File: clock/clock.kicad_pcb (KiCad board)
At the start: 2 copper layers, 100 x 50 mm, 22 parts, among them J1 USB_OTG, J2 Barrel_Jack, U1 iv12, U2 iv12, U3 iv12, U4 iv12, U5 STM32F103C8Tx, Y1 8Mhz, Y2 32.768khz

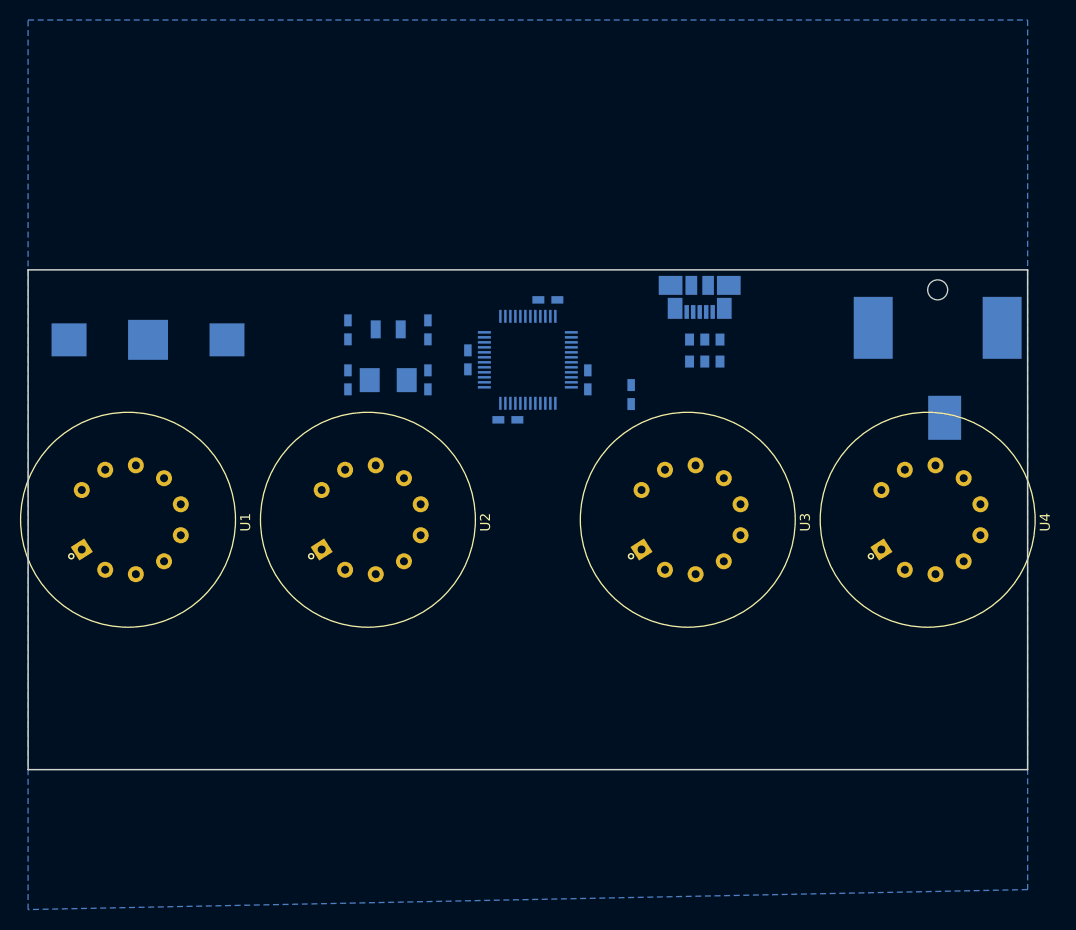
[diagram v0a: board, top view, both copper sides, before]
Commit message: Rev 1 of clock display board
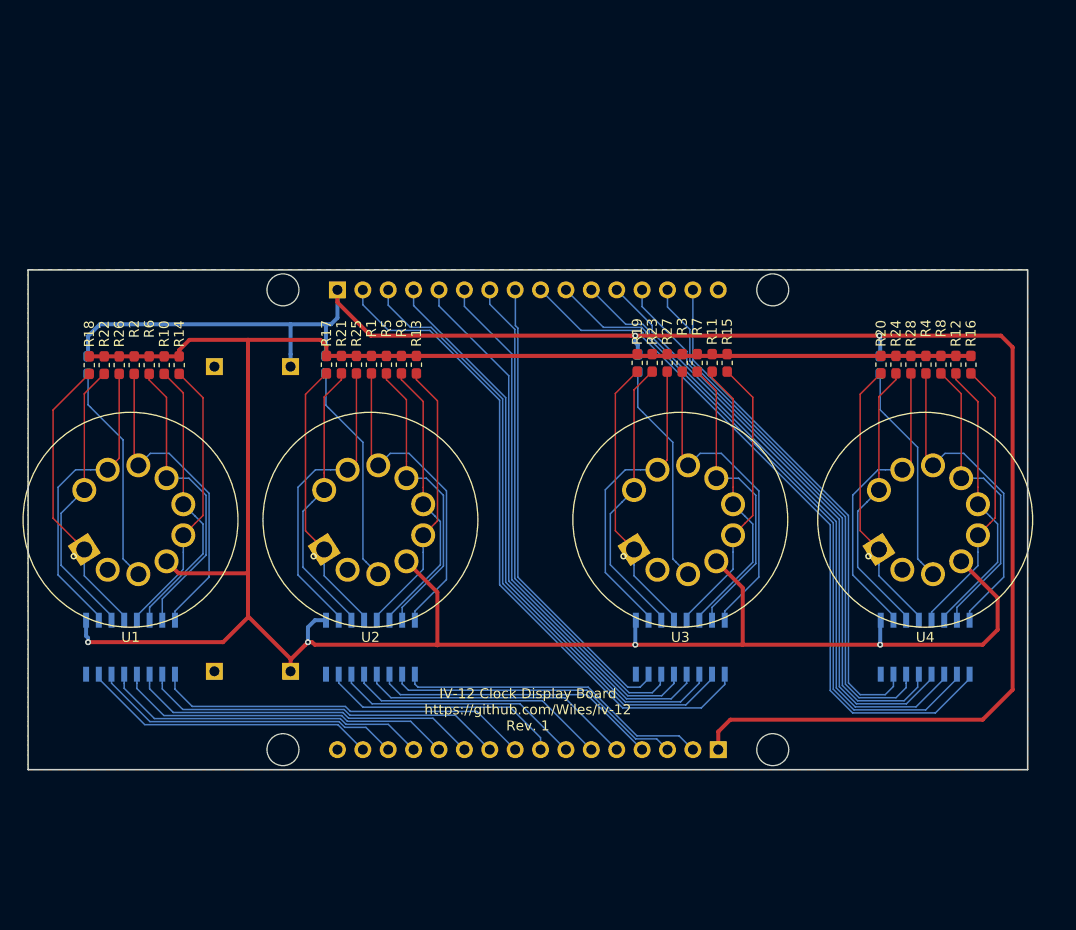
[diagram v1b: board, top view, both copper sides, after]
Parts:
- removed BT1: Battery_Cell, Battery_Holders:Keystone_3000_1x12mm-CoinCell
- removed C1, C2, C3, C4: 20p, Capacitors_SMD:C_0603_HandSoldering
- removed C5, C6, C7, C8, C9: 104, Capacitors_SMD:C_0603_HandSoldering
- removed Y1: 8Mhz, Crystals:Crystal_SMD_5032-2pin_5.0x3.2mm
- removed Y2: 32.768khz, Crystals:Crystal_SMD_3215-2pin_3.2x1.5mm
- added J3: 5v, Connector_PinHeader_2.54mm:PinHeader_1x01_P2.54mm_Vertical, B.Cu at (103.3, 111.7)
- added J4: Conn_01x01_Male, Connector_PinHeader_2.54mm:PinHeader_1x01_P2.54mm_Vertical, B.Cu at (95.6, 111.7)
- added J5: 24v, Connector_PinHeader_2.54mm:PinHeader_1x01_P2.54mm_Vertical, B.Cu at (103.3, 142.2)
- added J6: Conn_01x01_Male, Connector_PinHeader_2.54mm:PinHeader_1x01_P2.54mm_Vertical, B.Cu at (95.6, 142.2)
- added R10: 10k, Resistor_SMD:R_0603_1608Metric_Pad1.05x0.95mm_HandSolder, F.Cu at (90.6, 111.5)
- added R11: 10k, Resistor_SMD:R_0603_1608Metric_Pad1.05x0.95mm_HandSolder, F.Cu at (145.4, 111.3)
- added R12: 10k, Resistor_SMD:R_0603_1608Metric_Pad1.05x0.95mm_HandSolder, F.Cu at (169.8, 111.5)
- added R13: 10k, Resistor_SMD:R_0603_1608Metric_Pad1.05x0.95mm_HandSolder, F.Cu at (115.8, 111.5)
- added R14: 10k, Resistor_SMD:R_0603_1608Metric_Pad1.05x0.95mm_HandSolder, F.Cu at (92.1, 111.5)
- added R15: 10k, Resistor_SMD:R_0603_1608Metric_Pad1.05x0.95mm_HandSolder, F.Cu at (146.9, 111.3)
- added R16: 10k, Resistor_SMD:R_0603_1608Metric_Pad1.05x0.95mm_HandSolder, F.Cu at (171.3, 111.5)
- added R17: 10k, Resistor_SMD:R_0603_1608Metric_Pad1.05x0.95mm_HandSolder, F.Cu at (106.8, 111.5)
- added R18: 10k, Resistor_SMD:R_0603_1608Metric_Pad1.05x0.95mm_HandSolder, F.Cu at (83.1, 111.5)
- added R19: 10k, Resistor_SMD:R_0603_1608Metric_Pad1.05x0.95mm_HandSolder, F.Cu at (137.9, 111.3)
- added R20: 10k, Resistor_SMD:R_0603_1608Metric_Pad1.05x0.95mm_HandSolder, F.Cu at (162.3, 111.5)
- added R21: 10k, Resistor_SMD:R_0603_1608Metric_Pad1.05x0.95mm_HandSolder, F.Cu at (108.3, 111.5)
- added R22: 10k, Resistor_SMD:R_0603_1608Metric_Pad1.05x0.95mm_HandSolder, F.Cu at (84.6, 111.5)
- added R23: 10k, Resistor_SMD:R_0603_1608Metric_Pad1.05x0.95mm_HandSolder, F.Cu at (139.4, 111.3)
- added R24: 10k, Resistor_SMD:R_0603_1608Metric_Pad1.05x0.95mm_HandSolder, F.Cu at (163.8, 111.5)
- added R25: 10k, Resistor_SMD:R_0603_1608Metric_Pad1.05x0.95mm_HandSolder, F.Cu at (109.8, 111.5)
- added R26: 10k, Resistor_SMD:R_0603_1608Metric_Pad1.05x0.95mm_HandSolder, F.Cu at (86.1, 111.5)
- added R27: 10k, Resistor_SMD:R_0603_1608Metric_Pad1.05x0.95mm_HandSolder, F.Cu at (140.9, 111.3)
- added R28: 10k, Resistor_SMD:R_0603_1608Metric_Pad1.05x0.95mm_HandSolder, F.Cu at (165.3, 111.5)
- added R29: R_Small, Resistor_SMD:R_0603_1608Metric_Pad1.05x0.95mm_HandSolder, B.Cu at (138.0, 111.3)
- added R30: R_Small, Resistor_SMD:R_0603_1608Metric_Pad1.05x0.95mm_HandSolder, B.Cu at (106.8, 111.5)
- added R31: R_Small, Resistor_SMD:R_0603_1608Metric_Pad1.05x0.95mm_HandSolder, B.Cu at (83.0, 111.5)
- added R32: R_Small, Resistor_SMD:R_0603_1608Metric_Pad1.05x0.95mm_HandSolder, B.Cu at (162.2, 111.5)
- added R4: 10k, Resistor_SMD:R_0603_1608Metric_Pad1.05x0.95mm_HandSolder, F.Cu at (166.8, 111.5)
- added R5: 10k, Resistor_SMD:R_0603_1608Metric_Pad1.05x0.95mm_HandSolder, F.Cu at (112.8, 111.5)
- added R6: 10k, Resistor_SMD:R_0603_1608Metric_Pad1.05x0.95mm_HandSolder, F.Cu at (89.1, 111.5)
- added R7: 10k, Resistor_SMD:R_0603_1608Metric_Pad1.05x0.95mm_HandSolder, F.Cu at (143.9, 111.3)
- added R8: 10k, Resistor_SMD:R_0603_1608Metric_Pad1.05x0.95mm_HandSolder, F.Cu at (168.3, 111.5)
- added R9: 10k, Resistor_SMD:R_0603_1608Metric_Pad1.05x0.95mm_HandSolder, F.Cu at (114.3, 111.5)
- added REF**: OSHW-Symbol_13.4x12mm_SilkScreen, Symbol:OSHW-Symbol_13.4x12mm_SilkScreen, B.Cu at (127.0, 127.0)
- added REF**: MountingHole_3.2mm_M3, MountingHole:MountingHole_3.2mm_M3, F.Cu at (102.5, 150.0)
- added REF**: MountingHole_3.2mm_M3, MountingHole:MountingHole_3.2mm_M3, F.Cu at (151.5, 150.0)
- added REF**: MountingHole_3.2mm_M3, MountingHole:MountingHole_3.2mm_M3, F.Cu at (102.5, 104.0)
- added REF**: MountingHole_3.2mm_M3, MountingHole:MountingHole_3.2mm_M3, F.Cu at (151.5, 104.0)
- added U6: ULN2003, Package_SO:SOIC-16_3.9x9.9mm_P1.27mm, B.Cu at (111.2, 139.8)
- added U7: ULN2003, Package_SO:SOIC-16_3.9x9.9mm_P1.27mm, B.Cu at (142.2, 139.8)
- added U8: ULN2003, Package_SO:SOIC-16_3.9x9.9mm_P1.27mm, B.Cu at (166.8, 139.8)
- J1: value USB_OTG -> Conn_01x16_Male; footprint Connectors_USB:USB_Micro-B_Molex_47346-0001 -> Connector_PinHeader_2.54mm:PinHeader_1x16_P2.54mm_Vertical
- J2: value Barrel_Jack -> Conn_01x16_Male; footprint Connectors:Barrel_Jack_CUI_PJ-036AH-SMT -> Connector_PinHeader_2.54mm:PinHeader_1x16_P2.54mm_Vertical
- R1, R2: value 22R -> 10k; footprint Resistors_SMD:R_0603_HandSoldering -> Resistor_SMD:R_0603_1608Metric_Pad1.05x0.95mm_HandSolder; moved to F.Cu
- R3: footprint Resistors_SMD:R_0603_HandSoldering -> Resistor_SMD:R_0603_1608Metric_Pad1.05x0.95mm_HandSolder; moved to F.Cu
- U1, U2, U3, U4: footprint tubes:iv12 -> tubes:iv12-large
- U5: value STM32F103C8Tx -> ULN2003; footprint Housings_QFP:LQFP-48_7x7mm_Pitch0.5mm -> Package_SO:SOIC-16_3.9x9.9mm_P1.27mm
- moved J2 60.5 mm to (108.0, 104.0), turned to 270 degrees
- moved R2 55.6 mm to (87.6, 111.5)
- moved U5 49.1 mm to (87.2, 139.8), turned to 90 degrees
- moved J1 46.5 mm to (146.1, 150.0), turned to 90 degrees
- moved R1 33.4 mm to (111.3, 111.5)
- moved R3 3.98 mm to (142.4, 111.3)
- moved U3 0.75 mm to (142.2, 127.0)
- moved U1 0.25 mm to (87.2, 127.0)
- moved U2 0.25 mm to (111.2, 127.0)
- moved U4 0.25 mm to (166.8, 127.0)
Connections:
- J1 pad 4: GND -> Net-(J1-Pad4)
- J1 pad 5: GND -> Net-(J1-Pad5)
- J1 pad 6: GND -> Net-(J1-Pad6)
- J2 pad 1: (no net) -> +5V
- J2 pad 2: GND -> Net-(J2-Pad2)
- J2 pad 3: GND -> Net-(J2-Pad3)
- R1 pad 1: Net-(J1-Pad3) -> +24V
- R1 pad 2: D+ -> Net-(R1-Pad2)
- R2 pad 1: Net-(J1-Pad2) -> +24V
- R2 pad 2: D- -> Net-(R2-Pad2)
- R3 pad 1: +5V -> +24V
- R3 pad 2: D+ -> Net-(R3-Pad2)
- U1 pad 1: (no net) -> Net-(R18-Pad2)
- U1 pad 10: (no net) -> Net-(R22-Pad2)
- U1 pad 3: +1V5 -> Net-(R31-Pad1)
- U1 pad 5: (no net) -> Net-(R14-Pad2)
- U1 pad 6: (no net) -> Net-(R10-Pad2)
- U1 pad 7: (no net) -> Net-(R6-Pad2)
- U1 pad 8: (no net) -> Net-(R2-Pad2)
- U1 pad 9: (no net) -> Net-(R26-Pad2)
- U2 pad 1: (no net) -> Net-(R17-Pad2)
- U2 pad 10: (no net) -> Net-(R21-Pad2)
- U2 pad 3: +1V5 -> Net-(R30-Pad1)
- U2 pad 5: (no net) -> Net-(R13-Pad2)
- U2 pad 6: (no net) -> Net-(R9-Pad2)
- U2 pad 7: (no net) -> Net-(R5-Pad2)
- U2 pad 8: (no net) -> Net-(R1-Pad2)
- U2 pad 9: (no net) -> Net-(R25-Pad2)
- U3 pad 1: (no net) -> Net-(R19-Pad2)
- U3 pad 10: (no net) -> Net-(R23-Pad2)
- U3 pad 3: +1V5 -> Net-(R29-Pad1)
- U3 pad 5: (no net) -> Net-(R15-Pad2)
- U3 pad 6: (no net) -> Net-(R11-Pad2)
- U3 pad 7: (no net) -> Net-(R7-Pad2)
- U3 pad 8: (no net) -> Net-(R3-Pad2)
- U3 pad 9: (no net) -> Net-(R27-Pad2)
- U4 pad 1: (no net) -> Net-(R20-Pad2)
- U4 pad 10: (no net) -> Net-(R24-Pad2)
- U4 pad 3: +1V5 -> Net-(R32-Pad1)
- U4 pad 5: (no net) -> Net-(R16-Pad2)
- U4 pad 6: (no net) -> Net-(R12-Pad2)
- U4 pad 7: (no net) -> Net-(R8-Pad2)
- U4 pad 8: (no net) -> Net-(R4-Pad2)
- U4 pad 9: (no net) -> Net-(R28-Pad2)
- U5 pad 1: VBAT -> Net-(J1-Pad9)
- U5 pad 10: (no net) -> Net-(R26-Pad2)
- U5 pad 11: (no net) -> Net-(R22-Pad2)
- U5 pad 12: (no net) -> Net-(R18-Pad2)
- U5 pad 13: (no net) -> Net-(R14-Pad2)
- U5 pad 14: (no net) -> Net-(R10-Pad2)
- U5 pad 15: (no net) -> Net-(R6-Pad2)
- U5 pad 16: (no net) -> Net-(R2-Pad2)
- U5 pad 2: (no net) -> Net-(J1-Pad10)
- U5 pad 3: Net-(C3-Pad1) -> Net-(J1-Pad11)
- U5 pad 4: Net-(C4-Pad1) -> Net-(J1-Pad12)
- U5 pad 5: Net-(C1-Pad1) -> Net-(J1-Pad13)
- U5 pad 6: Net-(C2-Pad1) -> Net-(J1-Pad14)
- U5 pad 7: (no net) -> Net-(J1-Pad15)
- U5 pad 9: +3V3 -> +24V
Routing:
- net +24V: track 0.00 -> 261.8 mm, vias 0 -> 4
- net +5V: track 0.00 -> 179.9 mm, vias 0 -> 2
- net Net-(J2-Pad9): track 0.00 -> 72.3 mm
- net Net-(J2-Pad10): track 0.00 -> 68.2 mm
- net Net-(J2-Pad2): track 0.00 -> 67.2 mm
- net Net-(J2-Pad11): track 0.00 -> 64.2 mm
- net Net-(J2-Pad3): track 0.00 -> 62.8 mm
- net Net-(J2-Pad12): track 0.00 -> 60.3 mm
- net Net-(J2-Pad4): track 0.00 -> 59.1 mm
- net Net-(J2-Pad13): track 0.00 -> 58.0 mm
- net Net-(J2-Pad5): track 0.00 -> 56.3 mm
- net Net-(J2-Pad14): track 0.00 -> 55.2 mm
- net Net-(J2-Pad6): track 0.00 -> 53.4 mm
- net Net-(J2-Pad15): track 0.00 -> 52.3 mm
- net Net-(J2-Pad7): track 0.00 -> 50.6 mm
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- added copper zone on F.Cu, net GND
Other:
- net class 24v added: clearance 0.152, trace_width 0.4, via_dia 0.6, via_drill 0.3
- net class 5v added: clearance 0.152, trace_width 0.4, via_dia 0.6, via_drill 0.3
- board text added: "IV-12 Clock Display Board https://github.com/Wiles/iv-12 Rev. 1"
- board text added: "MT3608"
